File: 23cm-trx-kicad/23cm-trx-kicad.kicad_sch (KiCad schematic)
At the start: 23 parts, among them SW1 RotaryEncoder_Switch, U1 LCD 20x4, U2 L78L09_SOT89

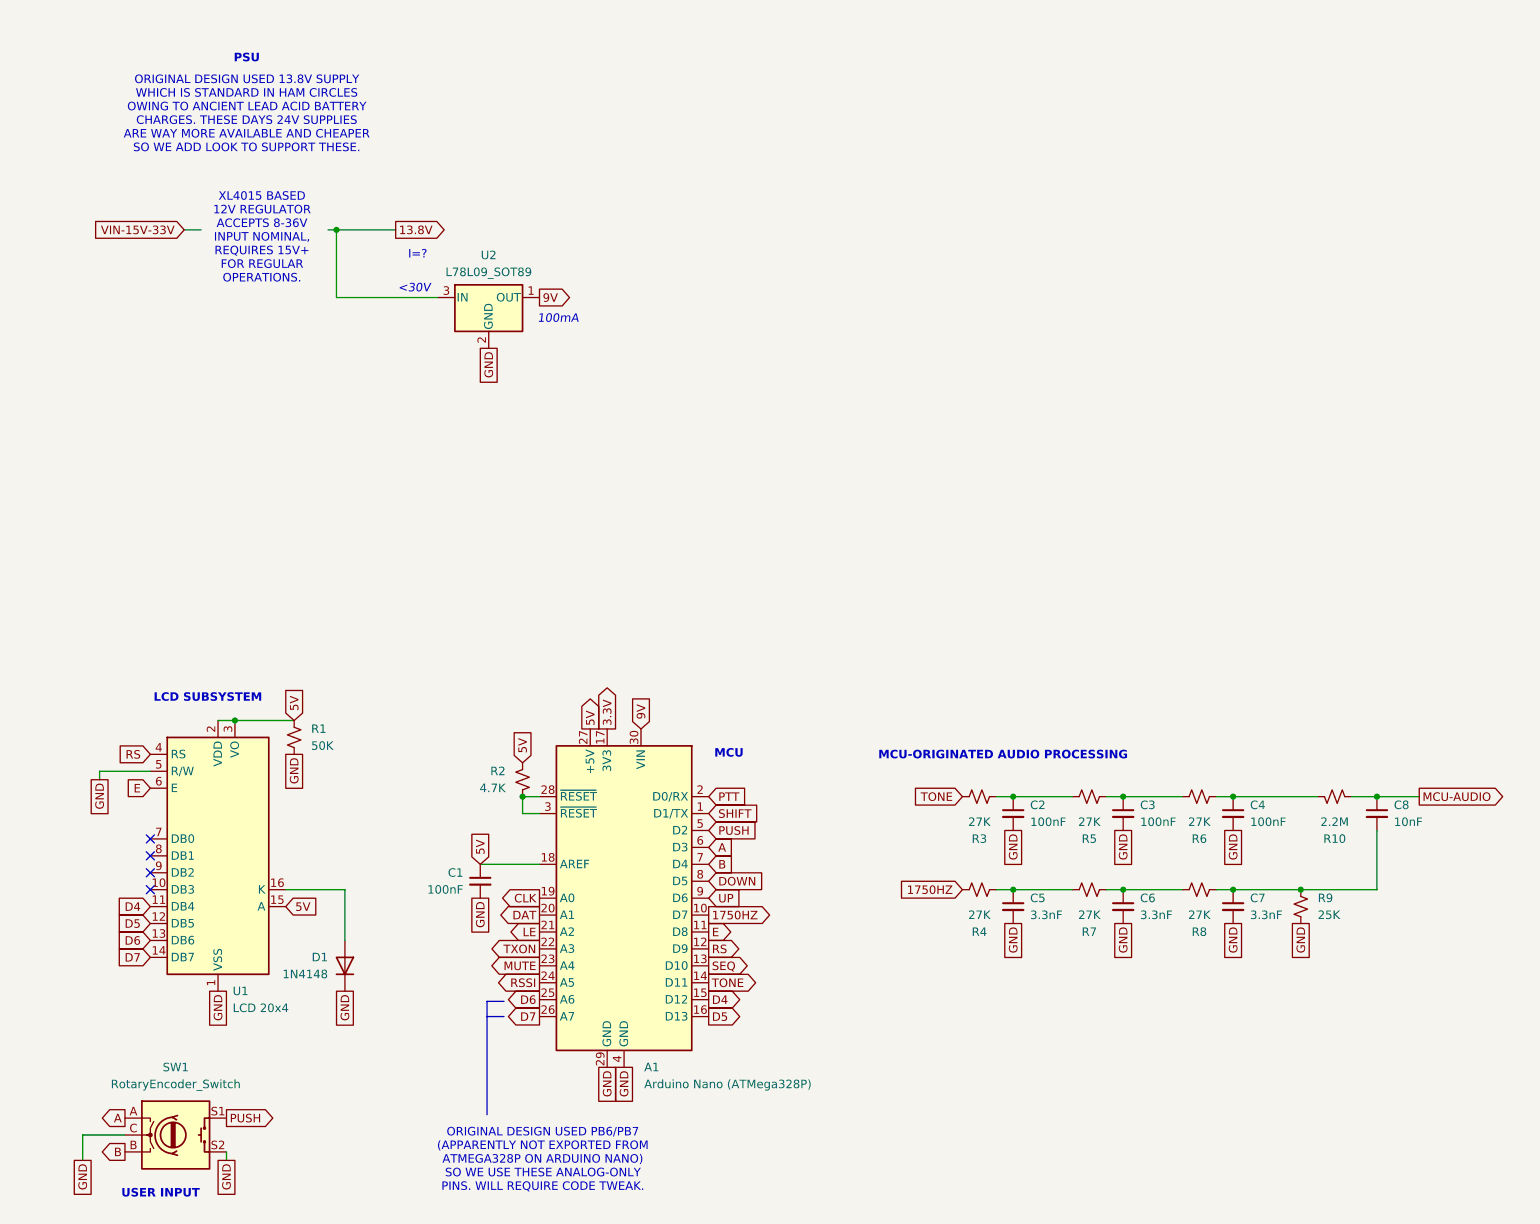
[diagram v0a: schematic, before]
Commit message: More schematic
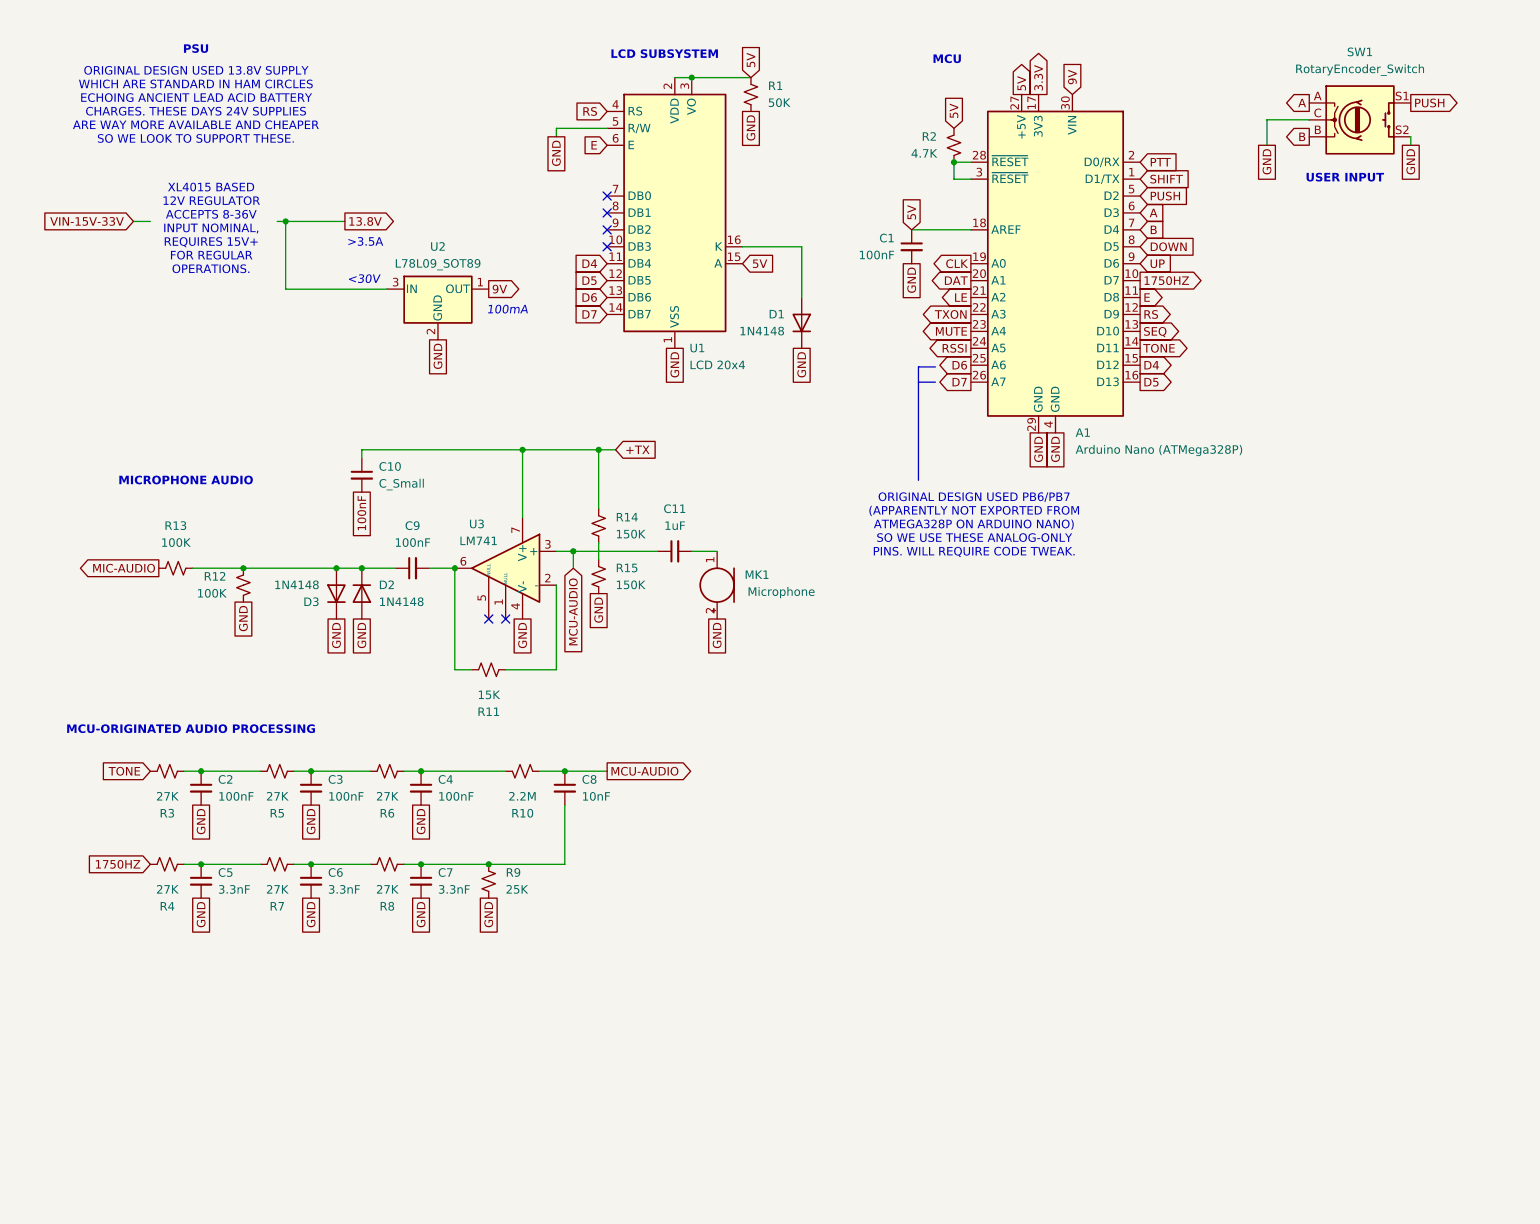
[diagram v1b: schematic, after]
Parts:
- added C10: C_Small, symbol Device:C_Small
- added C11: 1uF, symbol Device:C_Small
- added C9: 100nF, symbol Device:C_Small
- added D2, D3: 1N4148, Diode_THT:D_DO-35_SOD27_P7.62mm_Horizontal, symbol Diode:1N4148
- added MK1: Microphone, symbol Device:Microphone
- added R11: 15K, symbol Device:R_Small_US
- added R12, R13: 100K, symbol Device:R_Small_US
- added R14, R15: 150K, symbol Device:R_Small_US
- added U3: LM741, symbol Amplifier_Operational:LM741
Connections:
- net GND: now also D2.2 (A), D3.1 (K), MK1.2 (+), R12.2, R15.2, U3.4 (V-)
- net MCU-AUDIO: now also C11.1, U3.3 (+)
- new net: C9.1, D2.1 (K), D3.2 (A), R12.1, R13.2
- new net: C9.2, R11.1, U3.6
- new net: R14.2, R15.1
- new net: R11.2, U3.2 (-)
- new net: C11.2, MK1.1 (-)
- new net +TX: C10.1, R14.1, U3.7 (V+)
- new net 100nF: C10.2
- new net MIC-AUDIO: R13.1
- no-connect marks 4 -> 6
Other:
- note added: ">3.5A"
- note added: "MICROPHONE AUDIO"
- note added: "ORIGINAL DESIGN USED 13.8V SUPPLY WHICH ARE STANDARD IN HAM CIRCLES ECHOING ANCIENT LEAD ACID BATTERY CHARGES. THESE DAYS 24V SUPPLIES ARE WAY MORE AVAILABLE AND CHEAPER SO WE LOOK TO SUPPORT THESE."
- note removed: "I=?"
- note removed: "ORIGINAL DESIGN USED 13.8V SUPPLY WHICH IS STANDARD IN HAM CIRCLES OWING TO ANCIENT LEAD ACID BATTERY CHARGES. THESE DAYS 24V SUPPLIES ARE WAY MORE AVAILABLE AND CHEAPER SO WE ADD LOOK TO SUPPORT THESE."
- moved on the sheet: A1, C1, C2, C3, C4, C5, C6, C7, C8, D1, R1, R10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

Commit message: Further schematic work
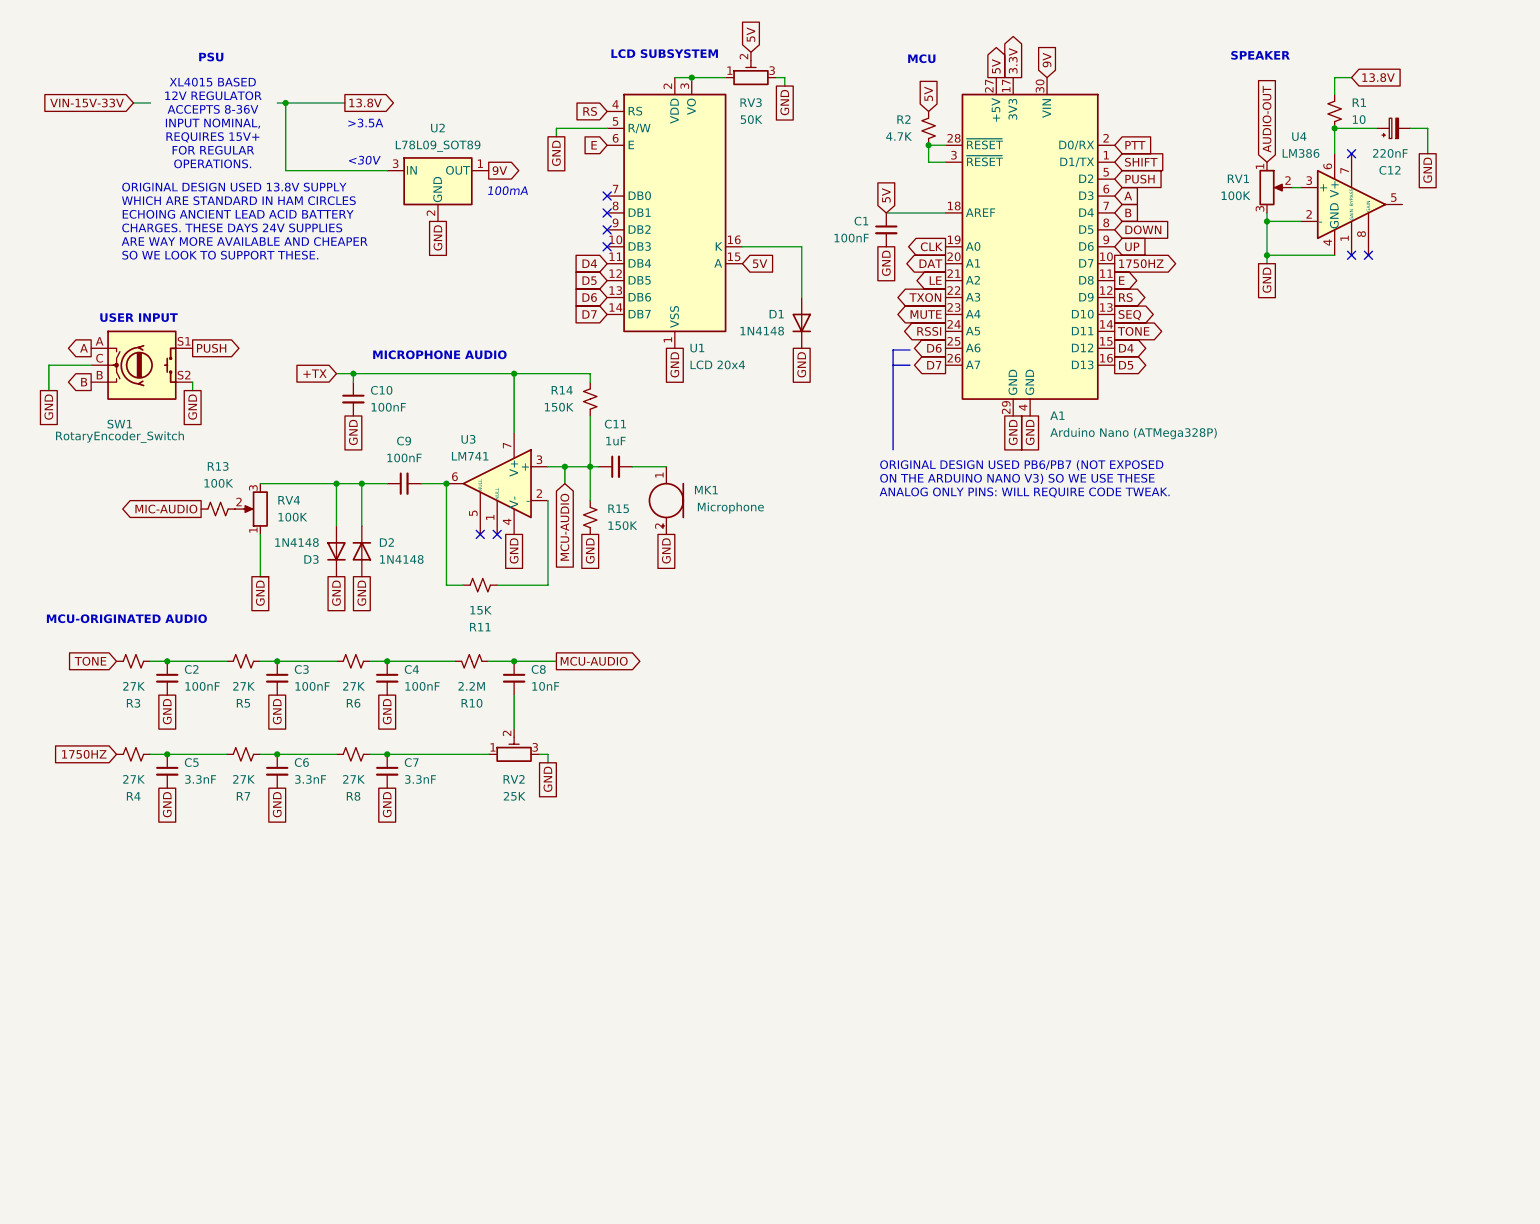
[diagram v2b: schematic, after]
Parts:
- removed R12: 100K, symbol Device:R_Small_US
- removed R9: 25K, symbol Device:R_Small_US
- added C12: 220nF, symbol Device:C_Polarized_Small
- added RV1, RV4: 100K, symbol Device:R_Potentiometer
- added RV2: 25K, symbol Device:R_Potentiometer_Trim
- added RV3: 50K, symbol Device:R_Potentiometer_Trim
- added U4: LM386, symbol Amplifier_Audio:LM386
- C10: value C_Small -> 100nF
- R1: value 50K -> 10
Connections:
- net 100nF is gone; now on net GND: C10.2
- net 13.8V: now also R1.1
- net 5V: now also RV3.2; no longer R1.1, U1.2 (VDD), U1.3 (VO)
- net GND: now also C12.2, RV1.3, RV2.3, RV3.3, RV4.1, U4.2 (-), U4.4 (GND); no longer R1.2
- net MCU-AUDIO: now also R14.2, R15.1
- net at C9.1, D2.1 (K), D3.2 (A): now also RV4.3; no longer R13.2
- net at C7.1, R8.2: now also RV2.1; no longer C8.2
- new net: C8.2, RV2.2
- new net: RV1.2, U4.3 (+)
- new net: C12.1, R1.2, U4.6 (V+)
- new net: RV3.1, U1.2 (VDD), U1.3 (VO)
- new net: R13.2, RV4.2
- new net AUDIO-OUT: RV1.1
- no-connect marks 6 -> 9
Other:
- note added: "MCU-ORIGINATED AUDIO"
- note added: "ORIGINAL DESIGN USED PB6/PB7 (NOT EXPOSED ON THE ARDUINO NANO V3) SO WE USE THESE ANALOG ONLY PINS: WILL REQUIRE CODE TWEAK."
- note added: "SPEAKER"
- note removed: "MCU-ORIGINATED AUDIO PROCESSING"
- note removed: "ORIGINAL DESIGN USED PB6/PB7 (APPARENTLY NOT EXPORTED FROM ATMEGA328P ON ARDUINO NANO) SO WE USE THESE ANALOG-ONLY PINS. WILL REQUIRE CODE TWEAK."
- moved on the sheet: A1, C1, C10, C11, C2, C3, C4, C5, C6, C7, C8, C9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
